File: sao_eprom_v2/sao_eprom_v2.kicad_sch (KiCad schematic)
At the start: 29 parts, among them J1 Conn_01x03, J2 USB_C_Receptacle_USB2.0, J3 sao_v2_addon_tht, U1 W25Q128JVS, U2 RP2040, U3 24LC00, X1 YSO110TR

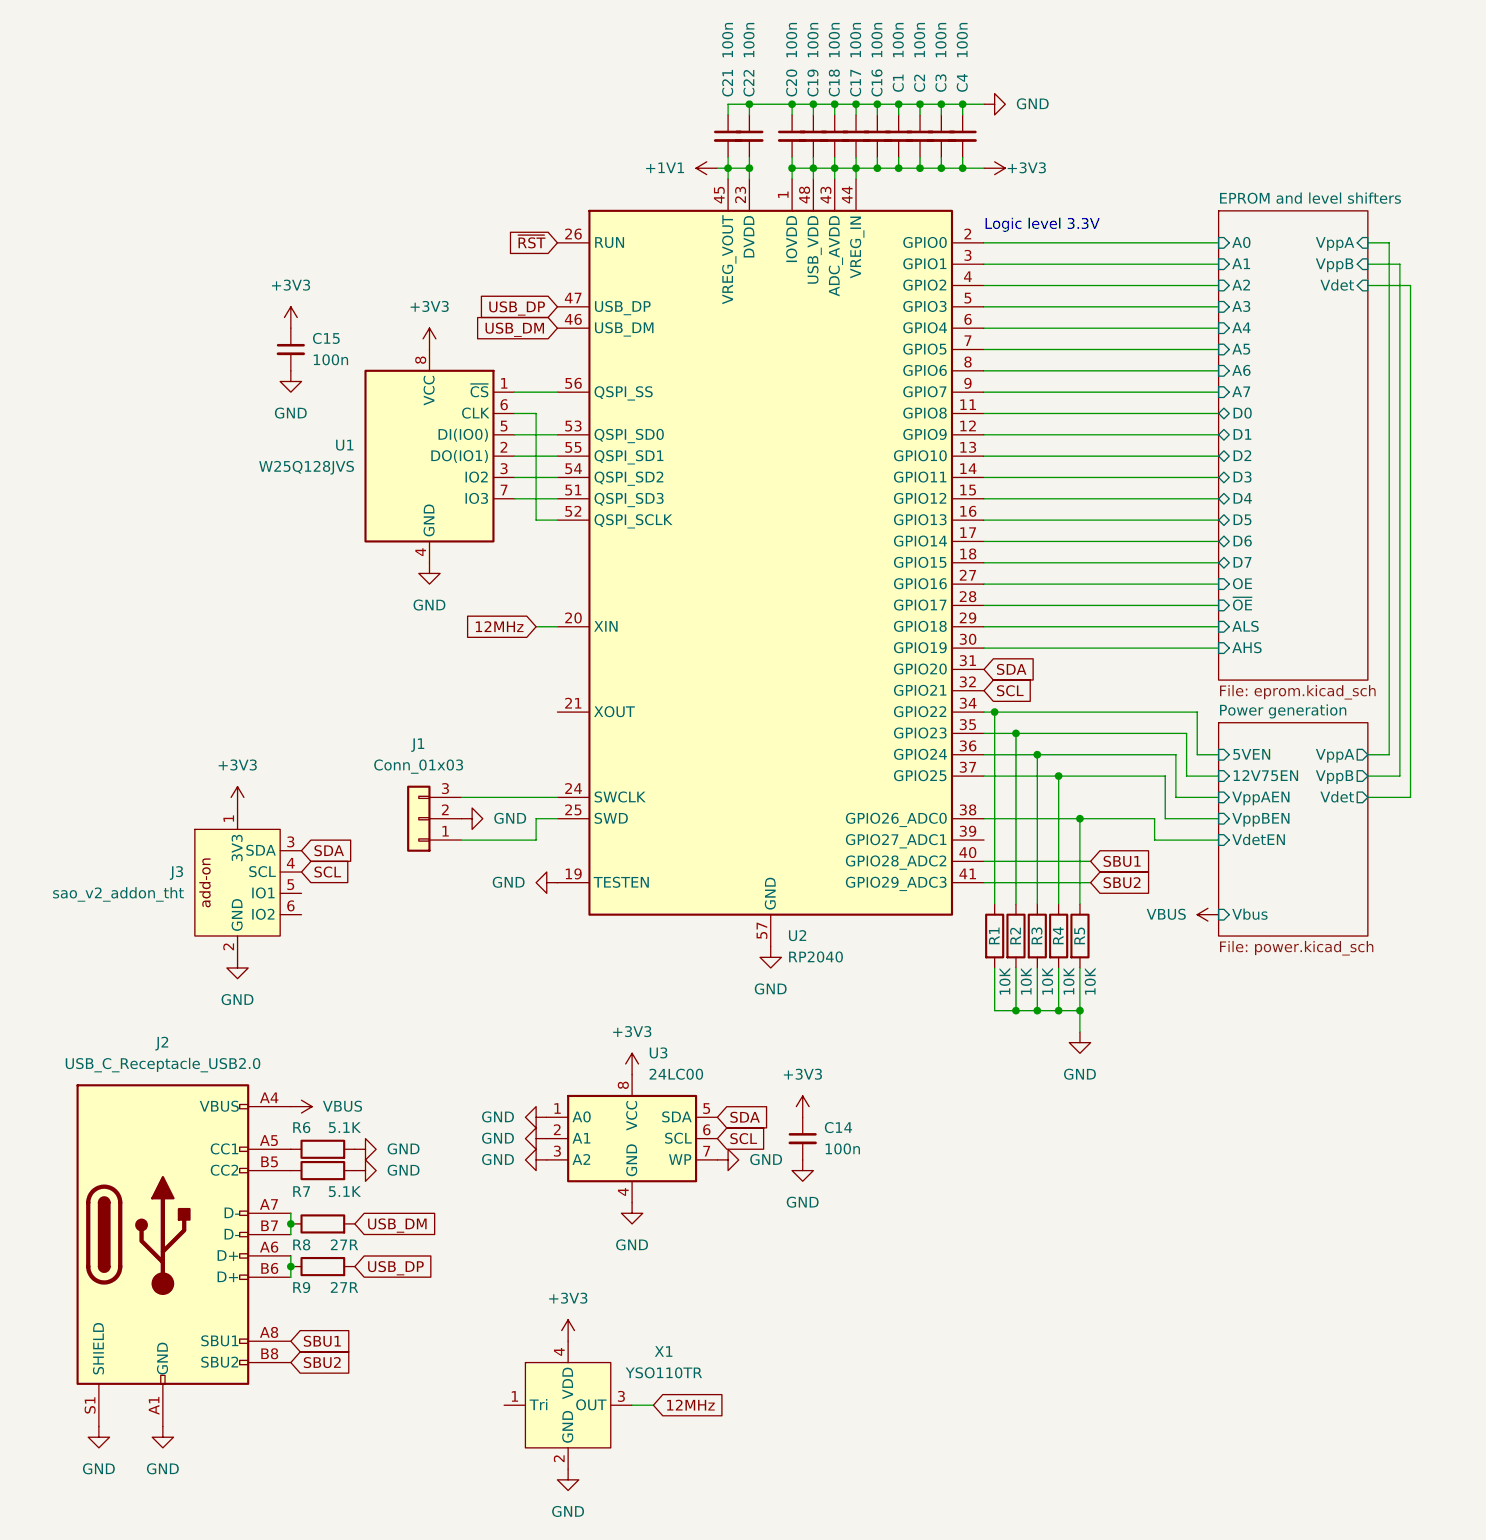
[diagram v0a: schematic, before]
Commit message: More tricky routing.
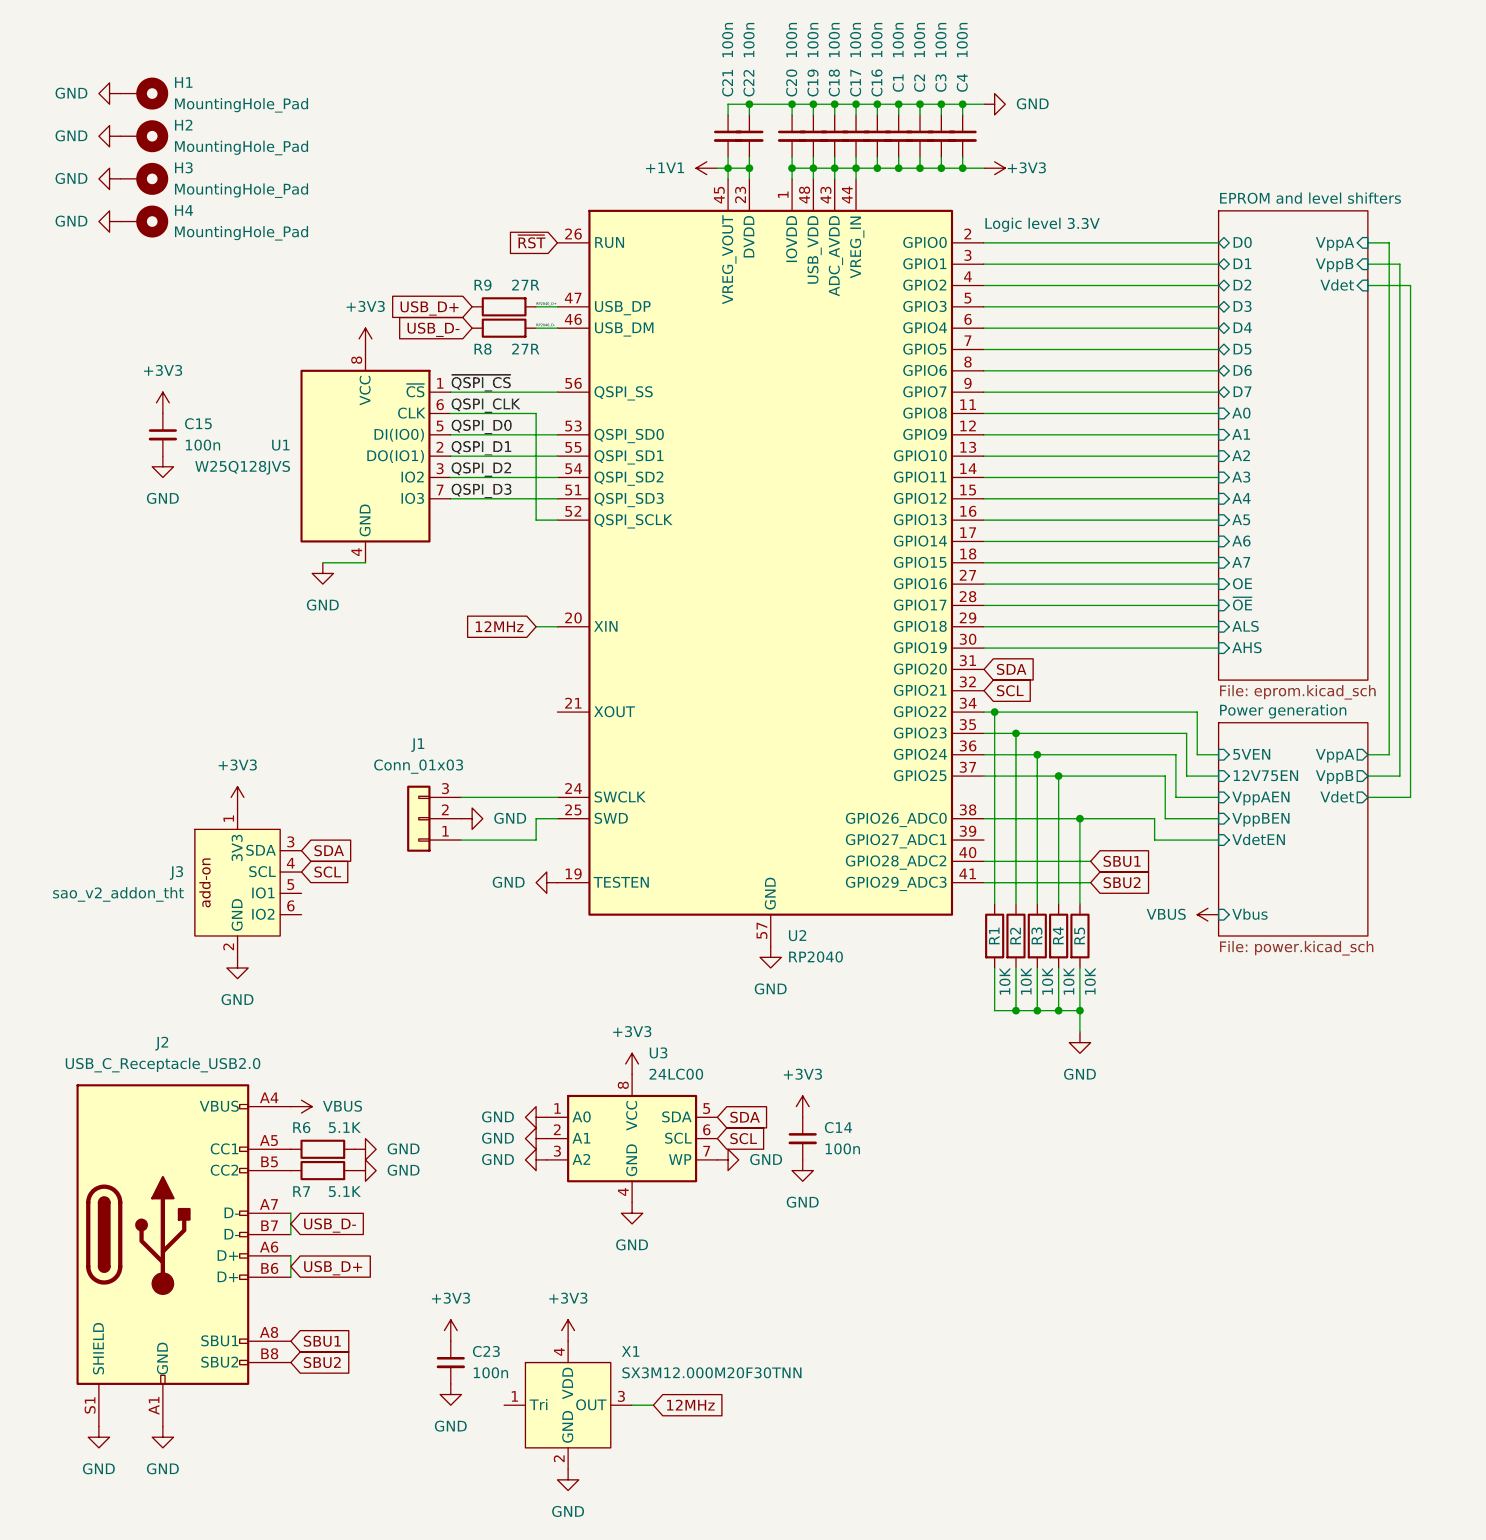
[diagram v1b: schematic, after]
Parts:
- added C23: 100n, Capacitor_SMD:C_0402_1005Metric_Pad0.74x0.62mm_HandSolder, symbol Device:C_Small
- added H1, H2, H3, H4: MountingHole_Pad, MountingHole:MountingHole_2.2mm_M2_Pad_Via, symbol Mechanical:MountingHole_Pad
- X1: value YSO110TR -> SX3M12.000M20F30TNN
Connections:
- net +3V3: now also C23.1
- net EPROM and level shifters/A0: now also U2.11 (GPIO8); no longer U2.2 (GPIO0)
- net EPROM and level shifters/A1: now also U2.12 (GPIO9); no longer U2.3 (GPIO1)
- net EPROM and level shifters/A2: now also U2.13 (GPIO10); no longer U2.4 (GPIO2)
- net EPROM and level shifters/A3: now also U2.14 (GPIO11); no longer U2.5 (GPIO3)
- net EPROM and level shifters/A4: now also U2.15 (GPIO12); no longer U2.6 (GPIO4)
- net EPROM and level shifters/A5: now also U2.16 (GPIO13); no longer U2.7 (GPIO5)
- net EPROM and level shifters/A6: now also U2.17 (GPIO14); no longer U2.8 (GPIO6)
- net EPROM and level shifters/A7: now also U2.18 (GPIO15); no longer U2.9 (GPIO7)
- net EPROM and level shifters/D0: now also U2.2 (GPIO0); no longer U2.11 (GPIO8)
- net EPROM and level shifters/D1: now also U2.3 (GPIO1); no longer U2.12 (GPIO9)
- net EPROM and level shifters/D2: now also U2.4 (GPIO2); no longer U2.13 (GPIO10)
- net EPROM and level shifters/D3: now also U2.5 (GPIO3); no longer U2.14 (GPIO11)
- net EPROM and level shifters/D4: now also U2.6 (GPIO4); no longer U2.15 (GPIO12)
- net EPROM and level shifters/D5: now also U2.7 (GPIO5); no longer U2.16 (GPIO13)
- net EPROM and level shifters/D6: now also U2.8 (GPIO6); no longer U2.17 (GPIO14)
- net EPROM and level shifters/D7: now also U2.9 (GPIO7); no longer U2.18 (GPIO15)
- net GND: now also C23.2, H1.1, H2.1, H3.1, H4.1
- net USB_D+: now reaches J2.A6 (D+), J2.B6 (D+), R9.1
- net USB_D-: now reaches J2.A7 (D-), J2.B7 (D-), R8.1
- net ~{QSPI_CS}: now reaches U1.1 (~{CS}), U2.56 (QSPI_SS)
- net QSPI_D1: now reaches U1.2 (DO(IO1)), U2.55 (QSPI_SD1)
- net QSPI_D2: now reaches U1.3 (IO2), U2.54 (QSPI_SD2)
- net QSPI_D0: now reaches U1.5 (DI(IO0)), U2.53 (QSPI_SD0)
- net QSPI_CLK: now reaches U1.6 (CLK), U2.52 (QSPI_SCLK)
- net QSPI_D3: now reaches U1.7 (IO3), U2.51 (QSPI_SD3)
- net USB_DM renamed RP2040_D-
- net USB_DP renamed RP2040_D+
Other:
- moved on the sheet: C15, R8, R9, U1

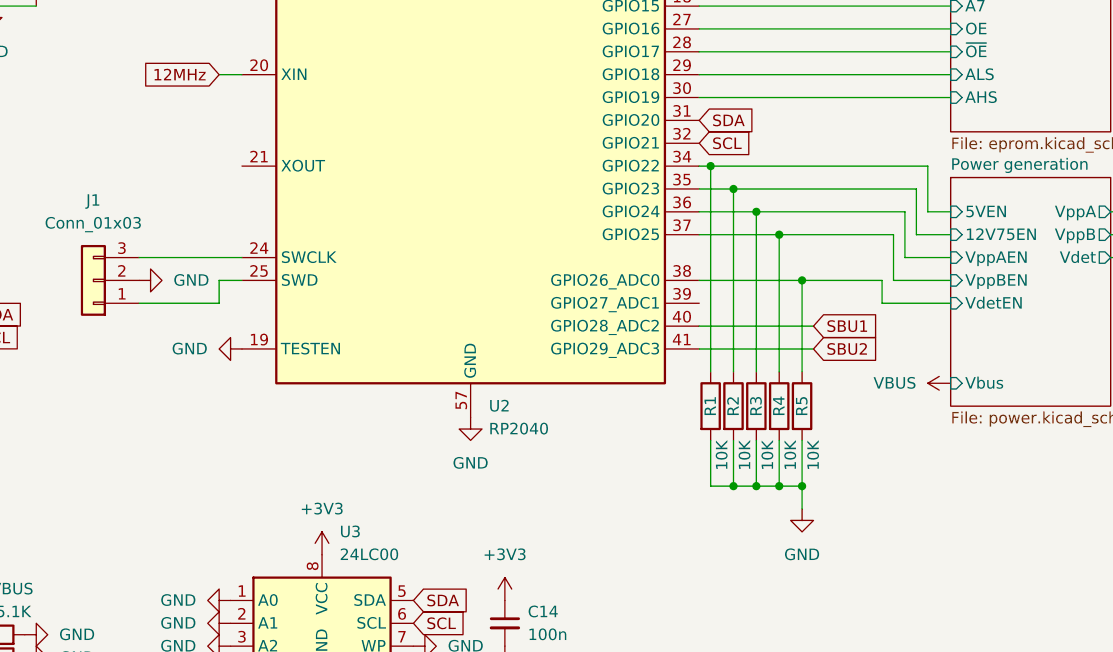
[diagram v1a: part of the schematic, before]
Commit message: Nearly finished the design
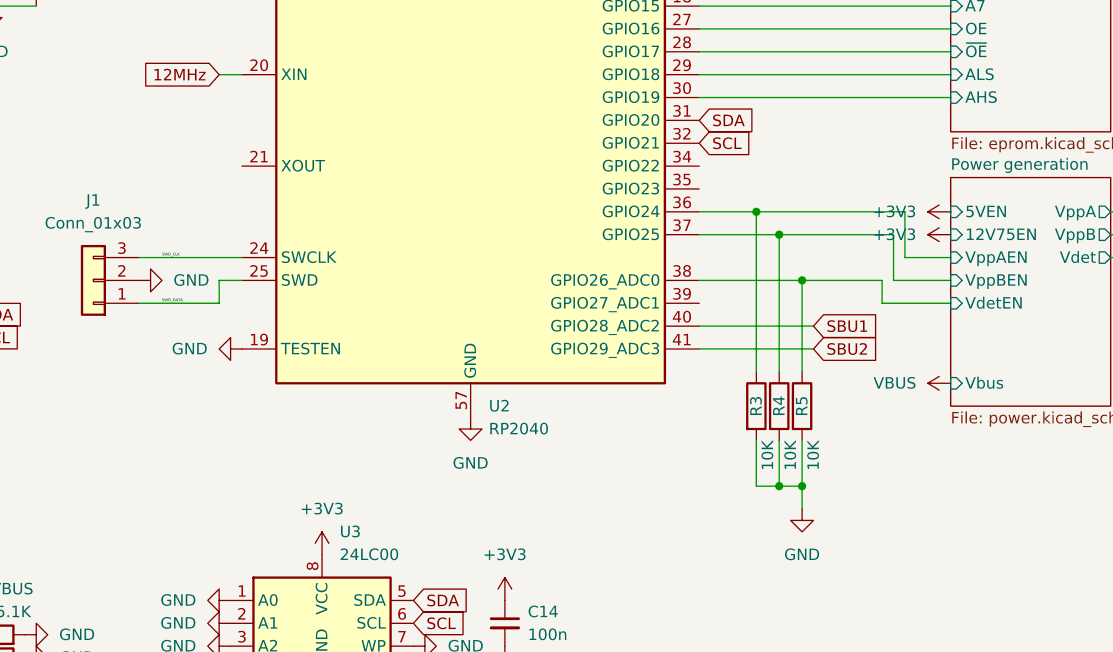
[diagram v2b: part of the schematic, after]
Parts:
- removed R1, R2: 10K, Resistor_SMD:R_0402_1005Metric_Pad0.72x0.64mm_HandSolder, symbol Device:R
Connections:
- net SWD_CLK: now reaches J1.3 (Pin_3), U2.24 (SWCLK)
- net SWD_DATA: now reaches J1.1 (Pin_1), U2.25 (SWD)
- net Power generation/12V75EN: no longer names the net of U2.35 (GPIO23)
- net Power generation/5VEN: no longer names the net of U2.34 (GPIO22)
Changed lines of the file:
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@@
   (junction (at 113.03 25.4) (diameter 0) (color 0 0 0 0)
   )
-  (junction (at 132.08 100.33) (diameter 0) (color 0 0 0 0)
-  )
   (junction (at 97.79 33.02) (diameter 0) (color 0 0 0 0)
   )
@@
   (junction (at 118.11 33.02) (diameter 0) (color 0 0 0 0)
   )
-  (junction (at 129.54 97.79) (diameter 0) (color 0 0 0 0)
-  )
   (junction (at 123.19 25.4) (diameter 0) (color 0 0 0 0)
   )
@@
   (junction (at 107.95 33.02) (diameter 0) (color 0 0 0 0)
   )
-  (junction (at 132.08 133.35) (diameter 0) (color 0 0 0 0)
-  )
   (junction (at 113.03 33.02) (diameter 0) (color 0 0 0 0)
   )
-  (junction (at 134.62 133.35) (diameter 0) (color 0 0 0 0)
-  )
   (junction (at 115.57 33.02) (diameter 0) (color 0 0 0 0)
   )
@@
     (stroke (width 0) (type default))
   )
-  (wire (pts (xy 132.08 100.33) (xy 152.4 100.33))
-    (stroke (width 0) (type default))
-  )
   (wire (pts (xy 139.7 110.49) (xy 128.27 110.49))
     (stroke (width 0) (type default))
@@
     (stroke (width 0) (type default))
   )
-  (wire (pts (xy 129.54 97.79) (xy 153.67 97.79))
-    (stroke (width 0) (type default))
-  )
   (wire (pts (xy 128.27 72.39) (xy 156.21 72.39))
     (stroke (width 0) (type default))
@@
     (stroke (width 0) (type default))
   )
-  (wire (pts (xy 132.08 100.33) (xy 132.08 120.65))
-    (stroke (width 0) (type default))
-  )
   (wire (pts (xy 128.27 44.45) (xy 156.21 44.45))
     (stroke (width 0) (type default))
@@
     (stroke (width 0) (type default))
   )
-  (wire (pts (xy 153.67 102.87) (xy 156.21 102.87))
-    (stroke (width 0) (type default))
-  )
   (wire (pts (xy 64.77 64.77) (xy 77.47 64.77))
     (stroke (width 0) (type default))
   )
-  (wire (pts (xy 153.67 97.79) (xy 153.67 102.87))
-    (stroke (width 0) (type default))
-  )
   (wire (pts (xy 139.7 133.35) (xy 137.16 133.35))
     (stroke (width 0) (type default))
@@
     (stroke (width 0) (type default))
   )
-  (wire (pts (xy 152.4 105.41) (xy 152.4 100.33))
-    (stroke (width 0) (type default))
-  )
   (wire (pts (xy 176.53 102.87) (xy 176.53 41.91))
     (stroke (width 0) (type default))
@@
     (stroke (width 0) (type default))
   )
-  (wire (pts (xy 128.27 97.79) (xy 129.54 97.79))
-    (stroke (width 0) (type default))
-  )
   (wire (pts (xy 123.19 33.02) (xy 125.73 33.02))
     (stroke (width 0) (type default))
@@
     (stroke (width 0) (type default))
   )
-  (wire (pts (xy 156.21 105.41) (xy 152.4 105.41))
-    (stroke (width 0) (type default))
-  )
   (wire (pts (xy 128.27 115.57) (xy 140.97 115.57))
     (stroke (width 0) (type default))
@@
     (stroke (width 0) (type default))
   )
-  (wire (pts (xy 132.08 133.35) (xy 134.62 133.35))
-    (stroke (width 0) (type default))
-  )
-  (wire (pts (xy 128.27 100.33) (xy 132.08 100.33))
-    (stroke (width 0) (type default))
-  )
   (wire (pts (xy 107.95 25.4) (xy 110.49 25.4))
     (stroke (width 0) (type default))
@@
     (stroke (width 0) (type default))
   )
-  (wire (pts (xy 129.54 133.35) (xy 132.08 133.35))
-    (stroke (width 0) (type default))
-  )
   (wire (pts (xy 128.27 54.61) (xy 156.21 54.61))
     (stroke (width 0) (type default))
@@
     (stroke (width 0) (type default))
   )
-  (wire (pts (xy 132.08 128.27) (xy 132.08 133.35))
-    (stroke (width 0) (type default))
-  )
   (wire (pts (xy 66.04 107.95) (xy 77.47 107.95))
     (stroke (width 0) (type default))
@@
     (stroke (width 0) (type default))
   )
-  (wire (pts (xy 129.54 128.27) (xy 129.54 133.35))
-    (stroke (width 0) (type default))
-  )
   (wire (pts (xy 74.93 62.23) (xy 74.93 74.93))
     (stroke (width 0) (type default))
@@
   )
   (wire (pts (xy 110.49 31.75) (xy 110.49 33.02))
-    (stroke (width 0) (type default))
-  )
-  (wire (pts (xy 129.54 97.79) (xy 129.54 120.65))
     (stroke (width 0) (type default))
   )
@@
     (effects (font (size 1.27 1.27)) (justify left bottom))
   )
+  (label "SWD_DATA" (at 68.58 113.03 0) (fields_autoplaced)
+    (effects (font (size 0.3 0.3)) (justify left bottom))
+  )
   (label "QSPI_D3" (at 64.77 72.39 0) (fields_autoplaced)
     (effects (font (size 1.27 1.27)) (justify left bottom))
+  )
+  (label "SWD_CLK" (at 68.58 107.95 0) (fields_autoplaced)
+    (effects (font (size 0.3 0.3)) (justify left bottom))
   )
   (label "QSPI_D1" (at 64.77 67.31 0) (fields_autoplaced)
@@
         (path "/07beccdd-32b3-4f03-aa51-fb5544b6f2d4"
           (reference "#PWR068") (unit 1)
+        )
+      )
+    )
+  )
+  (symbol (lib_id "power:+3V3") (at 156.21 102.87 90) (unit 1)
+    (in_bom yes) (on_board yes) (dnp no) (fields_autoplaced)
+    (property "Reference" "#PWR075" (at 160.02 102.87 0)
+      (effects (font (size 1.27 1.27)) hide)
+    )
+    (property "Value" "+3V3" (at 152.4 102.87 90)
+      (effects (font (size 1.27 1.27)) (justify left))
+    )
+    (property "Footprint" "" (at 156.21 102.87 0)
+      (effects (font (size 1.27 1.27)) hide)
+    )
+    (property "Datasheet" "" (at 156.21 102.87 0)
+      (effects (font (size 1.27 1.27)) hide)
+    )
+    (pin "1")
+    (instances
+      (project "sao_eprom_v2"
+        (path "/07beccdd-32b3-4f03-aa51-fb5544b6f2d4"
+          (reference "#PWR075") (unit 1)
         )
       )
@@
     )
   )
+  (symbol (lib_id "power:+3V3") (at 156.21 105.41 90) (unit 1)
+    (in_bom yes) (on_board yes) (dnp no) (fields_autoplaced)
+    (property "Reference" "#PWR076" (at 160.02 105.41 0)
+      (effects (font (size 1.27 1.27)) hide)
+    )
+    (property "Value" "+3V3" (at 152.4 105.41 90)
+      (effects (font (size 1.27 1.27)) (justify left))
+    )
+    (property "Footprint" "" (at 156.21 105.41 0)
+      (effects (font (size 1.27 1.27)) hide)
+    )
+    (property "Datasheet" "" (at 156.21 105.41 0)
+      (effects (font (size 1.27 1.27)) hide)
+    )
+    (pin "1")
+    (instances
+      (project "sao_eprom_v2"
+        (path "/07beccdd-32b3-4f03-aa51-fb5544b6f2d4"
+          (reference "#PWR076") (unit 1)
+        )
+      )
+    )
+  )
   (symbol (lib_id "Device:R") (at 71.12 52.07 90) (unit 1)
     (in_bom yes) (on_board yes) (dnp no)
@@
         (path "/07beccdd-32b3-4f03-aa51-fb5544b6f2d4"
           (reference "#PWR071") (unit 1)
-        )
-      )
-    )
-  )
-  (symbol (lib_id "Device:R") (at 129.54 124.46 0) (unit 1)
-    (in_bom yes) (on_board yes) (dnp no)
-    (property "Reference" "R1" (at 129.54 124.46 90)
-      (effects (font (size 1.27 1.27)))
-    )
-    (property "Value" "10K" (at 130.81 128.27 90)
-      (effects (font (size 1.27 1.27)) (justify right))
-    )
-    (property "Footprint" "Resistor_SMD:R_0402_1005Metric_Pad0.72x0.64mm_HandSolder" (at 127.762 124.46 90)
-      (effects (font (size 1.27 1.27)) hide)
-    )
-    (property "Datasheet" "~" (at 129.54 124.46 0)
-      (effects (font (size 1.27 1.27)) hide)
-    )
-    (pin "1")
-    (pin "2")
-    (instances
-      (project "sao_eprom_v2"
-        (path "/07beccdd-32b3-4f03-aa51-fb5544b6f2d4"
-          (reference "R1") (unit 1)
         )
       )
@@
         )
       )
-    )
-  )
-  (symbol (lib_id "Device:R") (at 132.08 124.46 0) (unit 1)
-    (in_bom yes) (on_board yes) (dnp no)
-    (property "Reference" "R2" (at 132.08 124.46 90)
-      (effects (font (size 1.27 1.27)))
-    )
-    (property "Value" "10K" (at 133.35 128.27 90)
-      (effects (font (size 1.27 1.27)) (justify right))
-    )
-    (property "Footprint" "Resistor_SMD:R_0402_1005Metric_Pad0.72x0.64mm_HandSolder" (at 130.302 124.46 90)
-      (effects (font (size 1.27 1.27)) hide)
-    )
-    (property "Datasheet" "~" (at 132.08 124.46 0)
-      (effects (font (size 1.27 1.27)) hide)
-    )
-    (pin "1")
-    (pin "2")
-    (instances
-      (project "sao_eprom_v2"
-        (path "/07beccdd-32b3-4f03-aa51-fb5544b6f2d4"
-          (reference "R2") (unit 1)
-        )
-      )
